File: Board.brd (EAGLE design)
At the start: 53.3 x 44.1 mm, 17 parts

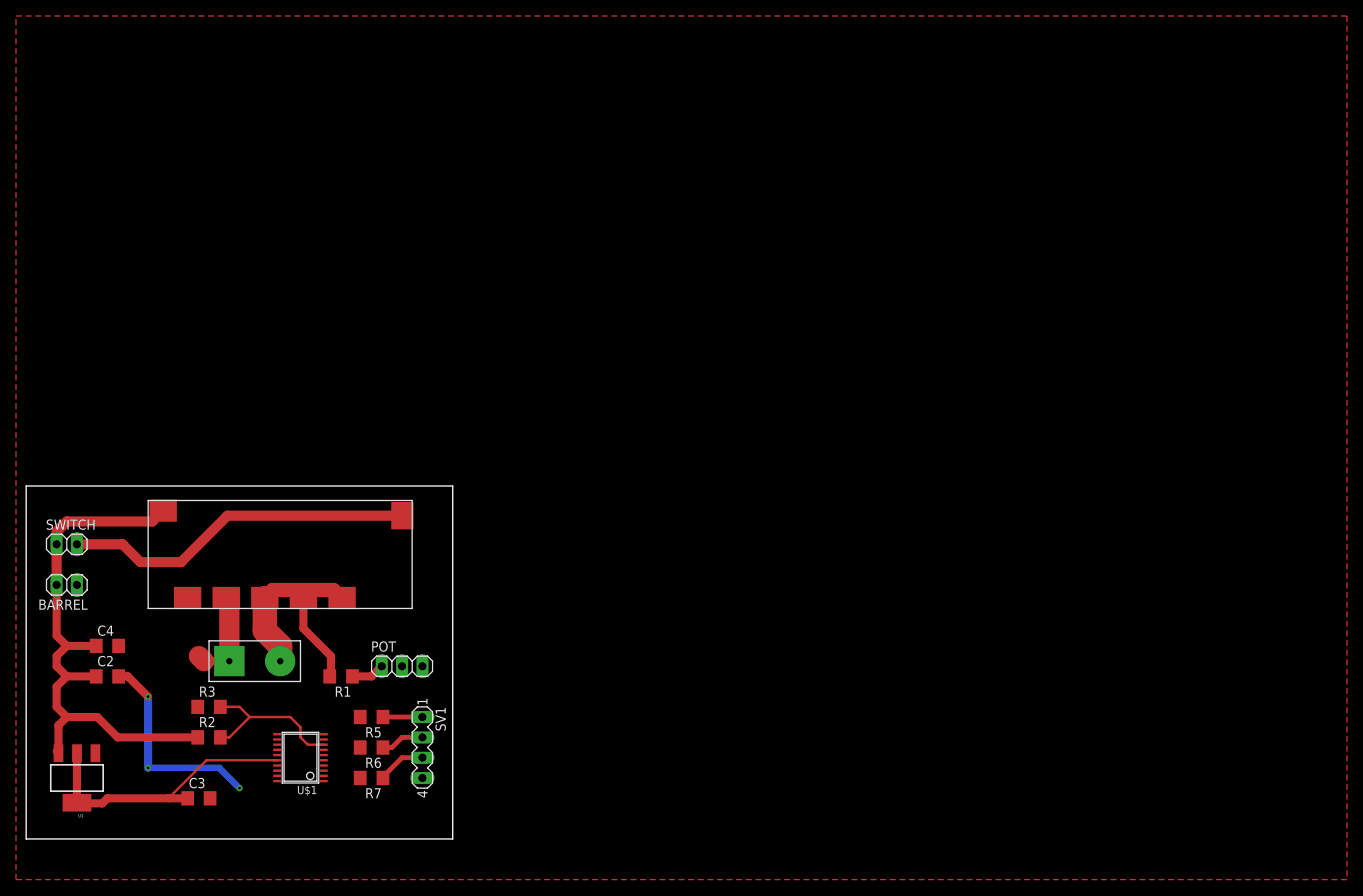
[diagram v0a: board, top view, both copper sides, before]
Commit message: Board design Rev1
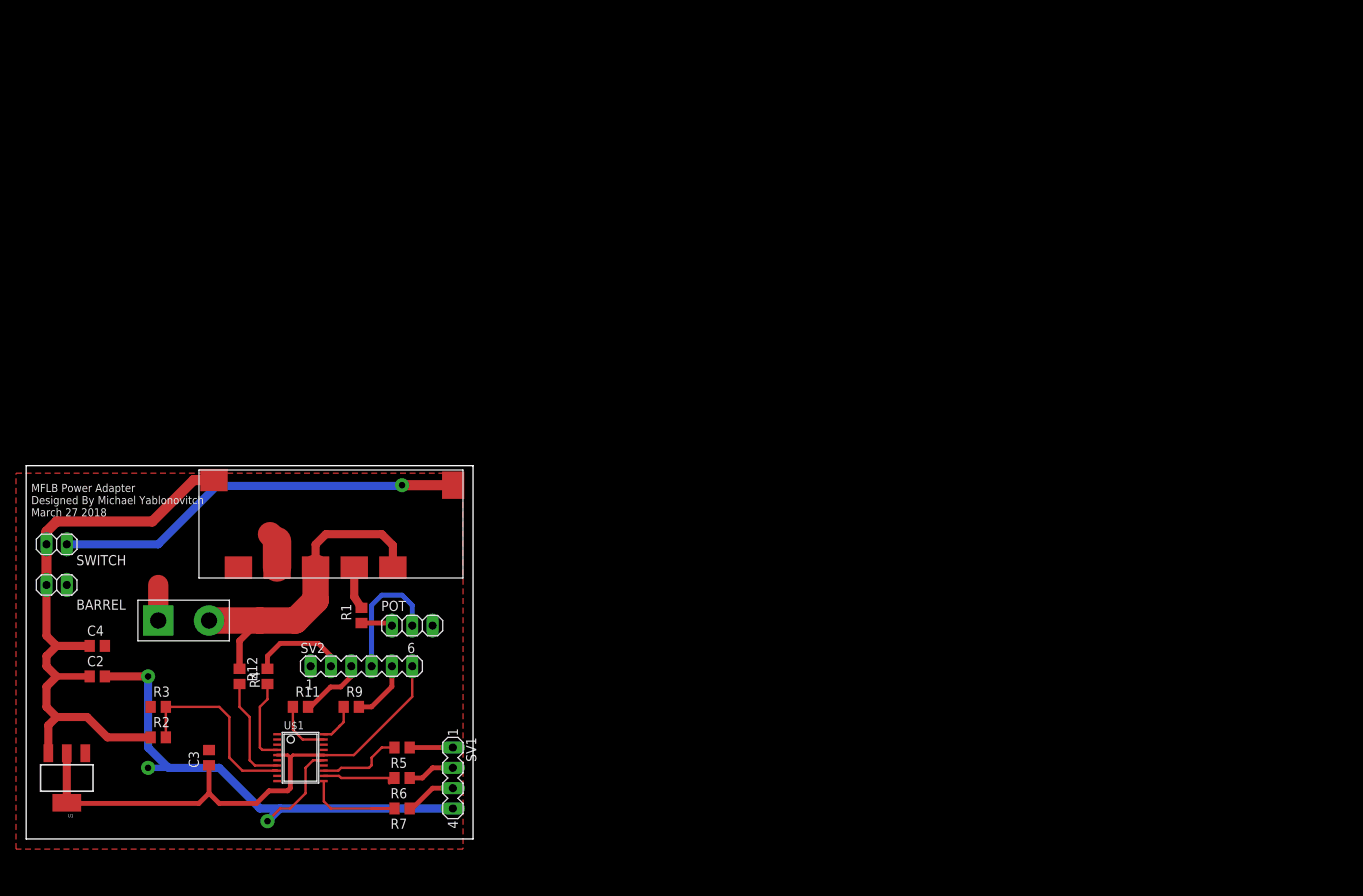
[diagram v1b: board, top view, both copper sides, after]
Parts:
- added R11, R12, R9: 250, rcl:R0805
- added R4: 1k, rcl:R0805
- added SV2: (no value), con-lstb:MA06-1
- C2, C3: value (none) -> 10uF; device rcl:C1206 -> rcl:C0805
- C4: value (none) -> 22uF; device rcl:C1206 -> rcl:C0805
- R1: value (none) -> 9.1k; device rcl:R1206 -> rcl:R0805
- R2: value (none) -> 7.5k; device rcl:R1206 -> rcl:R0805
- R3: value (none) -> 2.5k; device rcl:R1206 -> rcl:R0805
- R5, R6: value (none) -> 250; device rcl:R1206 -> rcl:R0805
- R7: value (none) -> 300; device rcl:R1206 -> rcl:R0805
- moved POWER 10.2 mm to (19.1, 27.3)
- moved R1 8.03 mm to (41.9, 27.9), turned to 90 degrees
- moved OKY-T/16-D12N-C 7.41 mm to (38.1, 39.4)
- moved R2 6.35 mm to (16.5, 12.7)
- moved R3 6.35 mm to (16.5, 16.5)
- moved R5 5.39 mm to (47.0, 11.4)
- moved R6 5.39 mm to (47.0, 7.62)
- moved R7 5.39 mm to (47.0, 3.81)
- moved SV1 5.39 mm to (53.3, 7.62)
- moved POT 5.24 mm to (48.3, 26.7)
- moved C3 5.24 mm to (22.9, 10.2), turned to 90 degrees
- moved BARREL 1.27 mm to (3.81, 31.8)
- moved SWITCH 1.27 mm to (3.81, 36.8)
- moved C2 1.27 mm to (8.89, 20.3)
- moved C4 1.27 mm to (8.89, 24.1)
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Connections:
- removed net N$2 (its old number): C3.1, U$1.16, U1.2, U1.4
- new net 3V3: C3.1, SV2.6, U$1.16, U$1.5, U1.2, U1.4
- new net N$19: R9.2, SV2.5
- new net N$21: R11.2, SV2.3
- new net N$22: R12.2, SV2.2
- new net N$9: R4.2, U$1.7
- new net NRST: R12.1, U$1.4
- new net SWCLK: R9.1, U$1.20
- new net SWDIO: R11.1, U$1.19
- new net SWO: SV2.1
- net GND: now also SV2.4, U$1.15
- net VOUT: now also R4.1; no longer U$1.7
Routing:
- net 3V3: track 0.00 -> 67.3 mm
- net GND: track 38.2 -> 98.1 mm
- net N$2 (its old number): track 35.9 -> 0.00 mm
- net VOUT: track 19.3 -> 42.9 mm
- net N$9: track 0.00 -> 13.8 mm
- net N$22: track 0.00 -> 13.4 mm
- net N$6: track 0.00 -> 11.7 mm
- net NRST: track 0.00 -> 10.6 mm
- net N$7: track 0.00 -> 10.6 mm
- net N$8: track 0.00 -> 10.1 mm
- net N$21: track 0.00 -> 8.70 mm
- net N$19: track 0.00 -> 7.72 mm
- net N$1: track 44.0 -> 51.4 mm, vias 0 -> 1
- net SWDIO: track 0.00 -> 7.23 mm
- net VIN: track 68.9 -> 75.6 mm
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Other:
- board size 53.3 x 44.1 mm -> 55.9 x 46.7 mm
- board text added: "MFLB Power Adapter Designed By Michael Yablonovitch March 27 2018"
